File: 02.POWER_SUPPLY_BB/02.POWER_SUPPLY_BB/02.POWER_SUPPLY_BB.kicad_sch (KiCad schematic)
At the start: 17 parts, among them J1 Conn_01x02_Pin, J2 Conn_01x02_Pin, J3 Conn_01x03_Pin, J4 Conn_01x03_Pin, J5 Screw_Terminal_01x02, J6 Barrel_Jack_Switch, J7 Screw_Terminal_01x02, U1 LM7806_TO220, U2 LM317_TO-220

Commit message: POWER_SUPPLY_BB - EESCHEMA - ASSOCIATE
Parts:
- C1, C2, C3: footprint (none) -> Capacitor_THT:C_Disc_D3.0mm_W1.6mm_P2.50mm
- D1: footprint (none) -> LED_THT:LED_D5.0mm
- J1, J2: footprint (none) -> Connector_PinHeader_2.54mm:PinHeader_1x02_P2.54mm_Vertical
- J3, J4: footprint (none) -> Connector_PinHeader_2.54mm:PinHeader_1x03_P2.54mm_Vertical
- J5, J7: footprint (none) -> TerminalBlock:TerminalBlock_bornier-2_P5.08mm
- J6: footprint (none) -> Connector_BarrelJack:BarrelJack_Horizontal
- R1, R2, R3: footprint (none) -> Resistor_THT:R_Axial_DIN0204_L3.6mm_D1.6mm_P7.62mm_Horizontal
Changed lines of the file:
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@@
 			)
 		)
-		(property "Footprint" ""
+		(property "Footprint" "Capacitor_THT:C_Disc_D3.0mm_W1.6mm_P2.50mm"
 			(at 125.4252 76.2 0)
 			(effects
@@
 			)
 		)
-		(property "Footprint" ""
+		(property "Footprint" "Resistor_THT:R_Axial_DIN0204_L3.6mm_D1.6mm_P7.62mm_Horizontal"
 			(at 89.662 139.7 90)
 			(effects
@@
 			)
 		)
-		(property "Footprint" ""
+		(property "Footprint" "LED_THT:LED_D5.0mm"
 			(at 74.93 135.89 0)
 			(effects
@@
 			)
 		)
-		(property "Footprint" ""
+		(property "Footprint" "Resistor_THT:R_Axial_DIN0204_L3.6mm_D1.6mm_P7.62mm_Horizontal"
 			(at 89.662 115.57 90)
 			(effects
@@
 			)
 		)
-		(property "Footprint" ""
+		(property "Footprint" "Capacitor_THT:C_Disc_D3.0mm_W1.6mm_P2.50mm"
 			(at 79.7052 76.2 0)
 			(effects
@@
 			)
 		)
-		(property "Footprint" ""
+		(property "Footprint" "Resistor_THT:R_Axial_DIN0204_L3.6mm_D1.6mm_P7.62mm_Horizontal"
 			(at 50.292 128.27 90)
 			(effects
@@
 			)
 		)
-		(property "Footprint" ""
+		(property "Footprint" "TerminalBlock:TerminalBlock_bornier-2_P5.08mm"
 			(at 223.52 132.08 0)
 			(effects
@@
 			)
 		)
-		(property "Footprint" ""
+		(property "Footprint" "Connector_PinHeader_2.54mm:PinHeader_1x03_P2.54mm_Vertical"
 			(at 218.44 55.88 0)
 			(effects
@@
 			)
 		)
-		(property "Footprint" ""
+		(property "Footprint" "Connector_BarrelJack:BarrelJack_Horizontal"
 			(at 29.21 70.866 0)
 			(effects
@@
 			)
 		)
-		(property "Footprint" ""
+		(property "Footprint" "Connector_PinHeader_2.54mm:PinHeader_1x02_P2.54mm_Vertical"
 			(at 219.71 121.92 0)
 			(effects
@@
 			)
 		)
-		(property "Footprint" ""
+		(property "Footprint" "TerminalBlock:TerminalBlock_bornier-2_P5.08mm"
 			(at 222.25 81.28 0)
 			(effects
@@
 			)
 		)
-		(property "Footprint" ""
+		(property "Footprint" "Capacitor_THT:C_Disc_D3.0mm_W1.6mm_P2.50mm"
 			(at 107.6452 120.65 0)
 			(effects
@@
 			)
 		)
-		(property "Footprint" ""
+		(property "Footprint" "Connector_PinHeader_2.54mm:PinHeader_1x02_P2.54mm_Vertical"
 			(at 218.44 72.39 0)
 			(effects
@@
 			)
 		)
-		(property "Footprint" ""
+		(property "Footprint" "Connector_PinHeader_2.54mm:PinHeader_1x03_P2.54mm_Vertical"
 			(at 219.71 107.95 0)
 			(effects

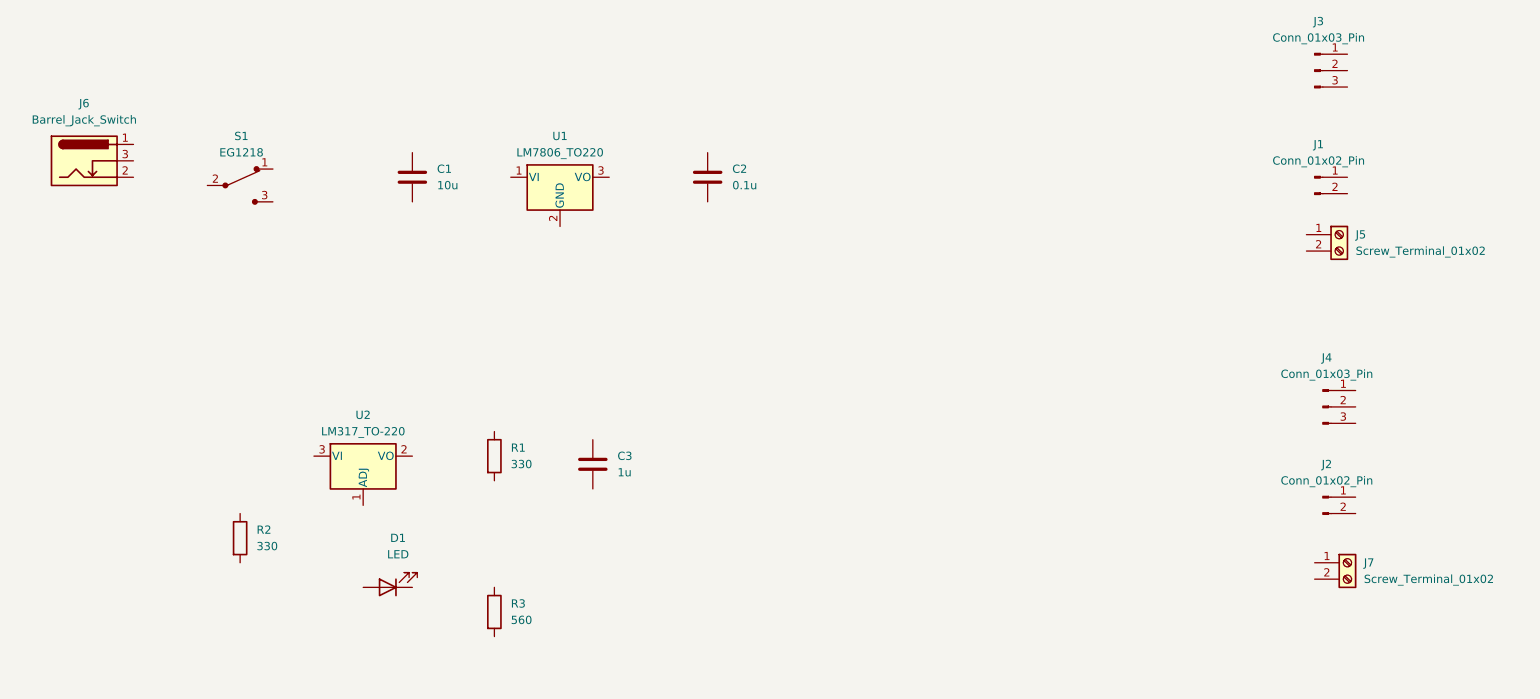
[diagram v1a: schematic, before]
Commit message: POWER_SUPPLY_BB - EESCHEMA - WIRING
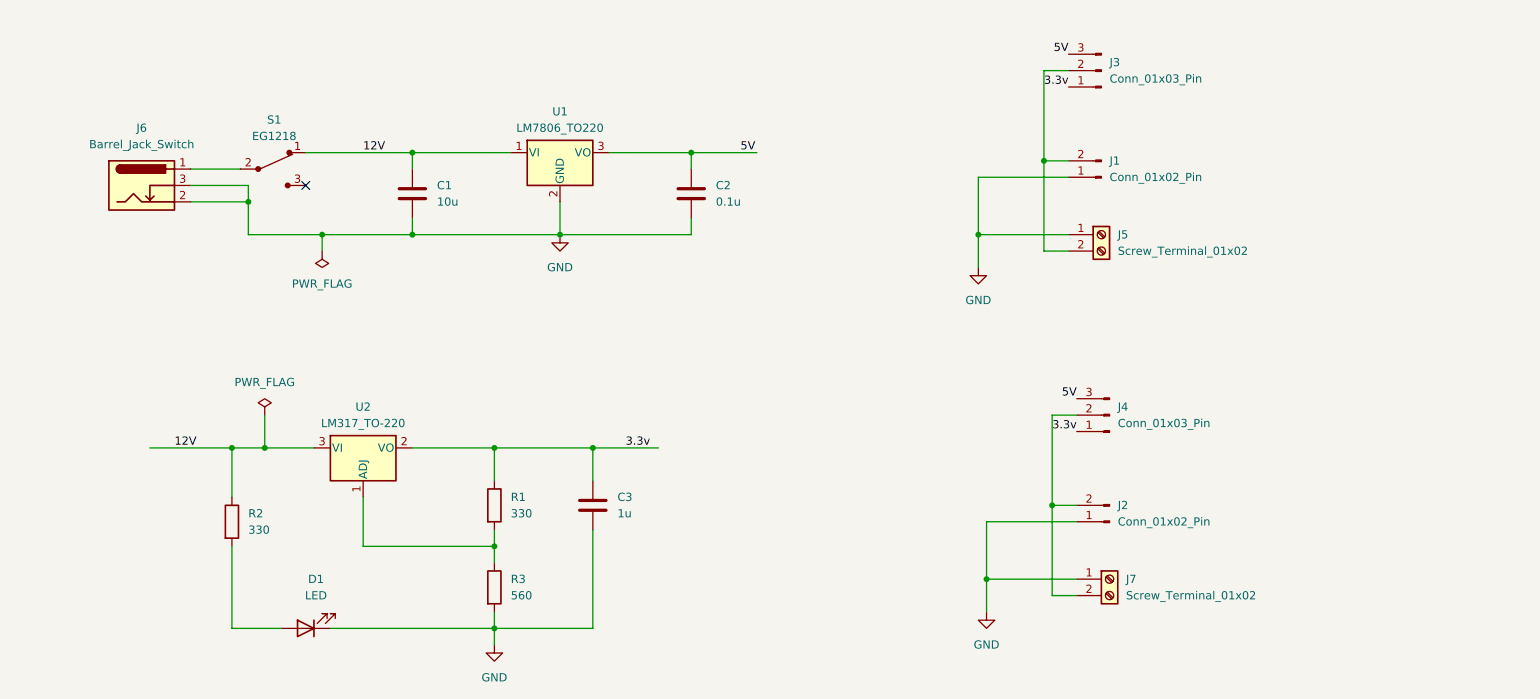
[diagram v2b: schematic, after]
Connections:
- net 5V: now reaches C2.1
- net 5V: now also J3.3 (Pin_3), J4.3 (Pin_3), U1.3 (VO)
- net GND: now reaches C2.2
- net GND: now also C1.2, C3.2, D1.1 (K), J1.1 (Pin_1), J2.1 (Pin_1), J5.1 (Pin_1), J6.2, J6.3, J7.1 (Pin_1), R3.2, U1.2 (GND)
- net at R3.1: now also R1.2, U2.1 (ADJ)
- net at D1.2 (A): now also R2.2
- net 3.3v: now reaches R1.1
- net 3.3v: now also C3.1, J3.1 (Pin_1), J4.1 (Pin_1), U2.2 (VO)
- net 12V: now reaches U2.3 (VI)
- net 12V: now also C1.1, R2.1, S1.1, U1.1 (VI)
- net at J7.2 (Pin_2): now also J2.2 (Pin_2), J4.2 (Pin_2)
- net at J3.2 (Pin_2): now also J1.2 (Pin_2), J5.2 (Pin_2)
- net at S1.2: now also J6.1
- no-connect marks 0 -> 1
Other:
- moved on the sheet: C1, C2, C3, D1, J1, J3, J5, J6, R1, R2, R3, S1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
